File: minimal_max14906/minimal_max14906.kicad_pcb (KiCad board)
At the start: 4 copper layers, 70.8 x 50.2 mm, 114 parts, among them J10 TBP02R2-381-02BE, J11 TBP02R2-381-02BE, J12 CLP-102-02-G-D-BE, J13 CLP-108-02-G-D-BE, J14 CLP-108-02-G-D-BE, J15 CLP-102-02-G-D-BE, J2 TBP02R2-381-02BE, J3 TBP02R2-381-02BE, J4 CLP-102-02-G-D-BE, J5 CLP-102-02-G-D-BE, J6 CLP-102-02-G-D-BE, J7 CLP-102-02-G-D-BE, J8 CLP-102-02-G-D-BE, Q1 -60.0 V, Q2 -60.0 V, Q3 -60.0 V, Q4 -60.0 V, Q5 100 V, Q6 100 V, U1 ADUM1252AUA+, U2 MAX22441CAEE+, U3 MAX22442CAEE+, U4 ADUM1252AUA+, U5 MAX14906ATM+, U6 ADUM1252AUA+

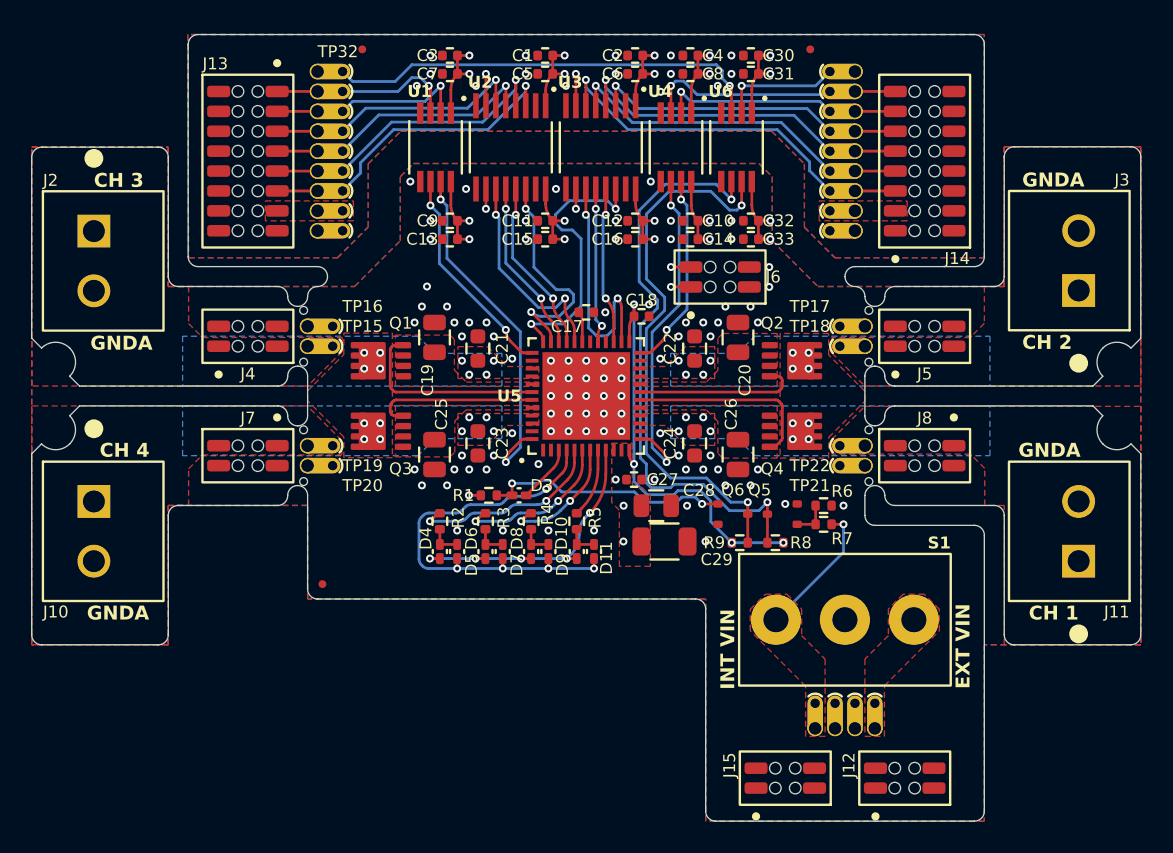
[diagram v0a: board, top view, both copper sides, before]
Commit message: development backup
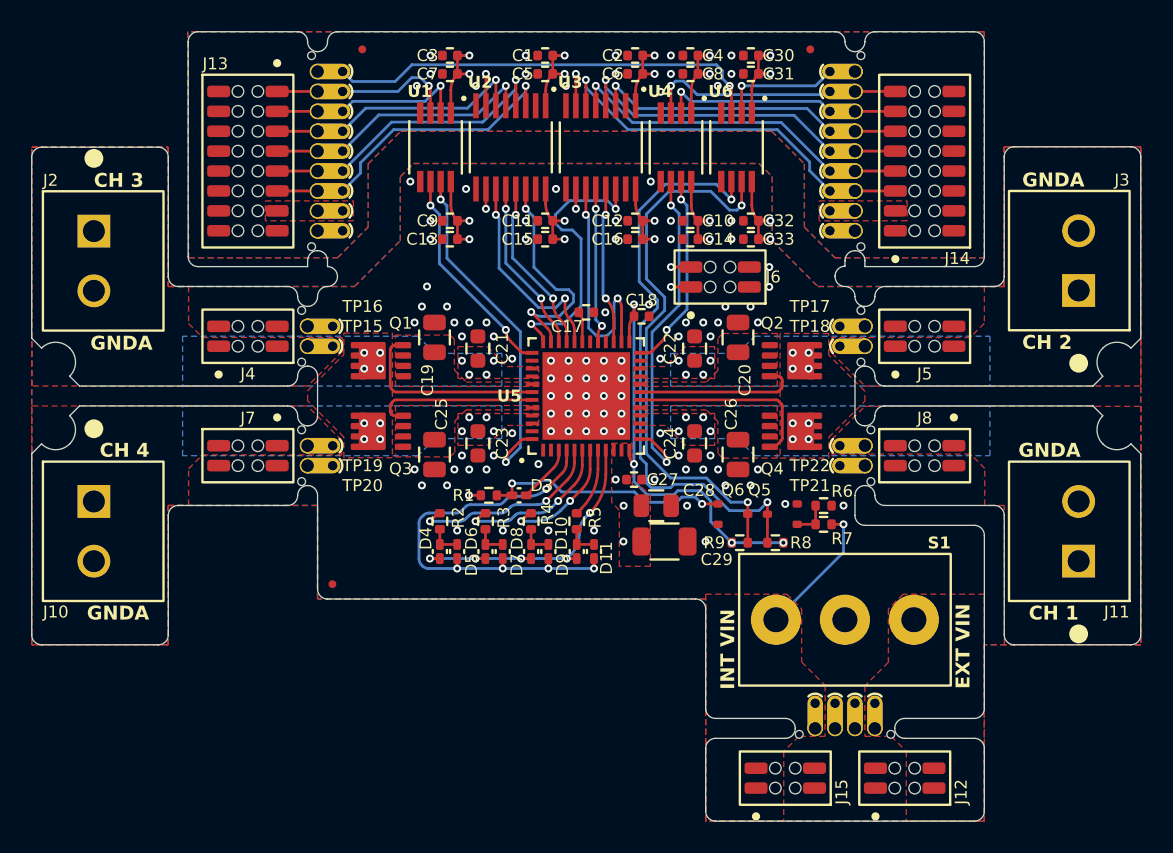
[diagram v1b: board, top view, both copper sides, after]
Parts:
- added MB1: mouse-bite-50mil-550mil, mouse_bite_footprints:mouse-bite-50mil-550mil, F.Cu at (118.1, 87.8)
- added MB6: mouse-bite-50mil-550mil, mouse_bite_footprints:mouse-bite-50mil-550mil, F.Cu at (152.4, 87.8)
- added MB8: mouse-bite-50mil-300mil, mouse_bite_footprints:mouse-bite-50mil-300mil, F.Cu at (151.8, 124.6)
- moved MB3 1.27 mm to (152.4, 99.6), turned to 90 degrees
- moved FID2 0.63 mm to (119.1, 115.4)
- moved MB2 0.63 mm to (117.5, 99.6), turned to -90 degrees
- moved MB4 0.63 mm to (117.5, 107.2), turned to -90 degrees
- moved MB5 0.63 mm to (153.0, 107.2), turned to 90 degrees
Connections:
- D4 pad 1: /SLED -> unconnected-(D4-Pad1)
- D5 pad 2: Net-(D4-Pad2) -> unconnected-(D5-Pad2)
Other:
- board size 70.8 x 50.2 mm -> 70.8 x 50.4 mm
